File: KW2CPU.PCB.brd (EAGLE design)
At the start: 50 x 30 mm, 57 parts, among them IC1 AT45DB161D8S1

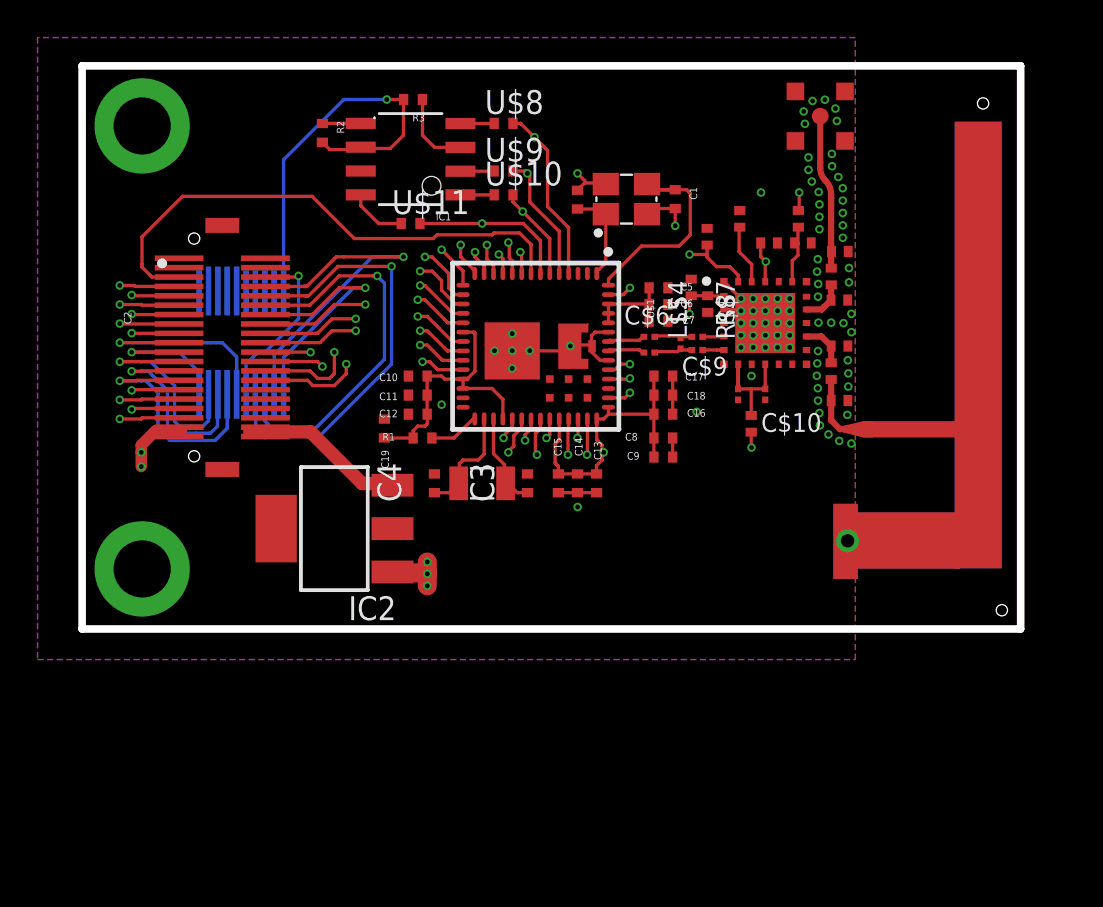
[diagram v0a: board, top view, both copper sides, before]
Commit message: Rotated board
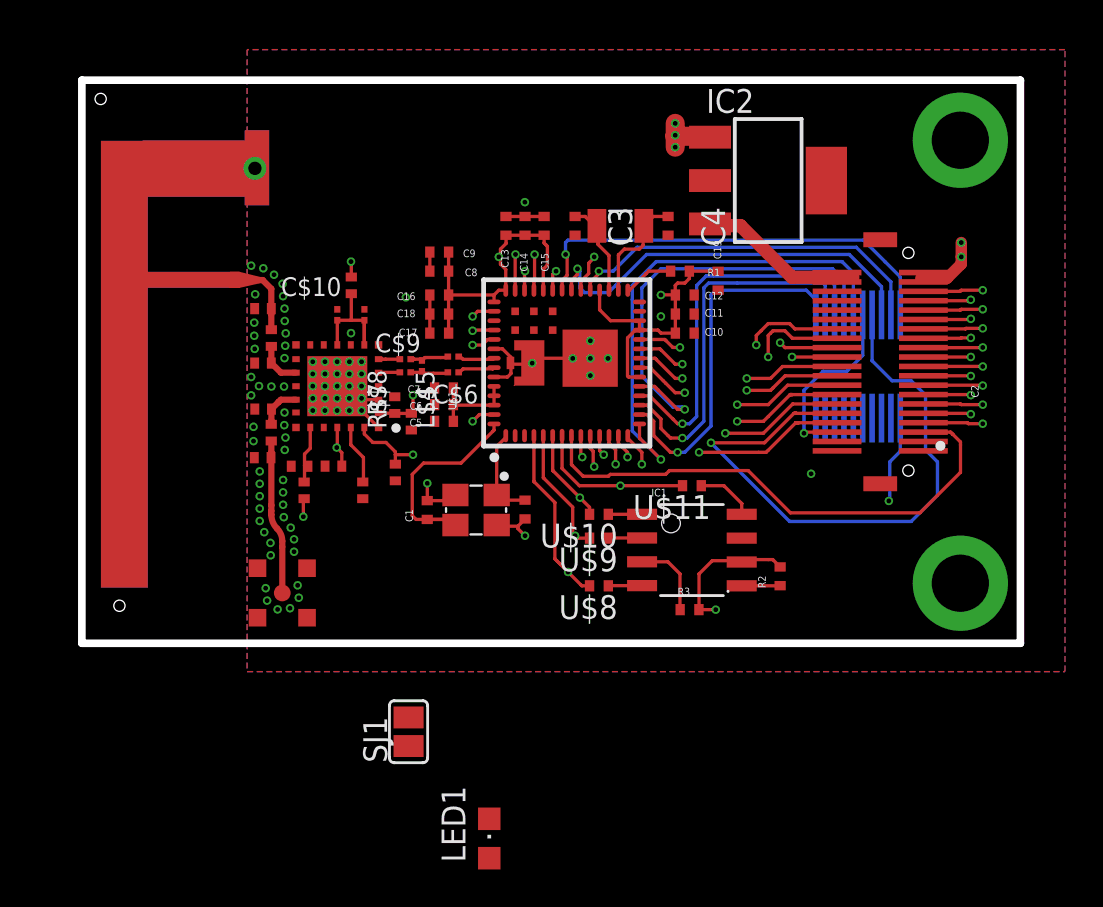
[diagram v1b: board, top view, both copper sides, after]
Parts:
- added LED1: (no value), adafruit:CHIPLED_0805
- added SJ1: (no value), jumper:SJ
- moved U$4 40.8 mm to (-3.79, 6.27), turned to 180 degrees
- moved U$5 38.3 mm to (1.16, -13.1), turned to 180 degrees
- moved U$6 35.1 mm to (33.0, -0.76), turned to 270 degrees
- moved R2 33.9 mm to (27.7, -12.2), turned to 90 degrees
- moved U$12 32.9 mm to (31.8, -1.01)
- moved C$16 32.7 mm to (0.12, -5.87), turned to 180 degrees
- moved C$18 31.2 mm to (0.14, -3.28), turned to 180 degrees
- moved C$15 31.1 mm to (0.14, 2.07), turned to 180 degrees
- moved L$17 31.0 mm to (0.58, -4.54), turned to 90 degrees
- moved R3 30.9 mm to (22.9, -14.0), turned to 0 degrees
- moved C$13 30.7 mm to (0.14, -0.83), turned to 180 degrees
- moved R$19 30.0 mm to (2.33, -7.61), turned to 270 degrees
- moved L$14 29.9 mm to (0.58, 0.50), turned to 90 degrees
- moved IC2 29.6 mm to (27.1, 8.89), turned to 270 degrees
- moved C$20 29.3 mm to (2.09, -6.33), turned to 0 degrees
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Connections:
- net GND: now also R$23.P$2
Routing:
- net N$22: track 37.7 -> 6.80 mm, vias 1 -> 0
- net N$40: track 38.2 -> 54.4 mm
- net N$13: track 33.1 -> 46.6 mm
- net N$41: track 33.6 -> 44.4 mm
- net N$44: track 34.4 -> 45.2 mm
- net N$11: track 40.0 -> 50.1 mm
- net N$43: track 31.8 -> 40.2 mm
- net +3V3: track 65.0 -> 56.7 mm, vias 10 -> 12
- net N$42: track 38.6 -> 46.7 mm
- net N$10: track 34.5 -> 41.9 mm
- net N$12: track 38.9 -> 45.1 mm
- net N$14: track 36.5 -> 37.2 mm
- net GND: vias 83 -> 84
